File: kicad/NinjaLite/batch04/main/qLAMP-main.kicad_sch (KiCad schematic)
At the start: 19 parts, among them J3 Conn_01x07_Male, J5 Conn_01x01_Male, Q3 Q_NMOS_GSD, Q5 Q_NMOS_GSD, U17 LITE_LCD, U5 ESP32-WROOM-32

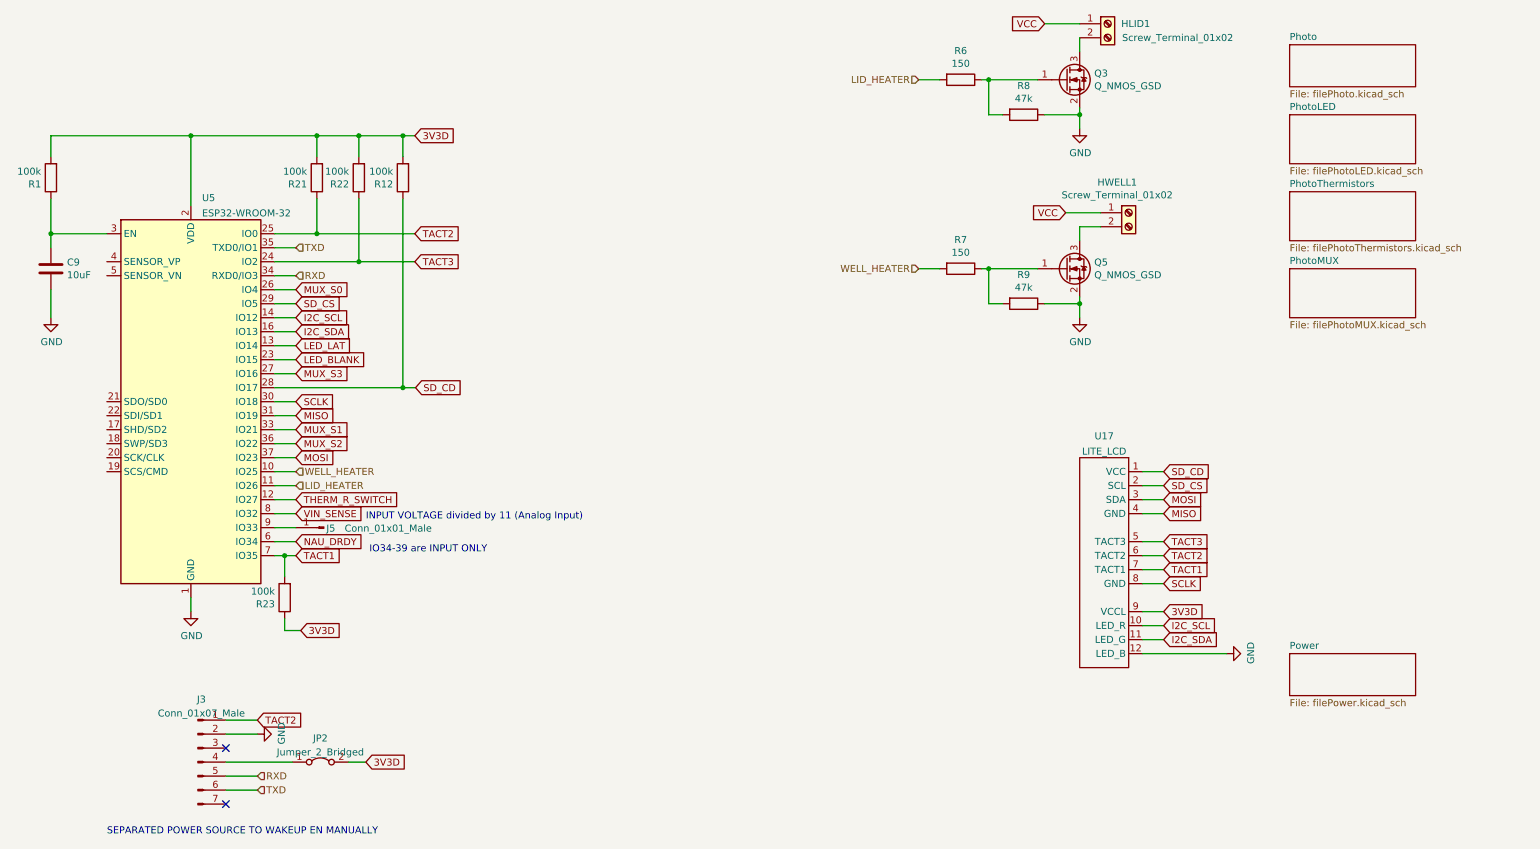
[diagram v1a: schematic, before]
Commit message: wiring batch04/main
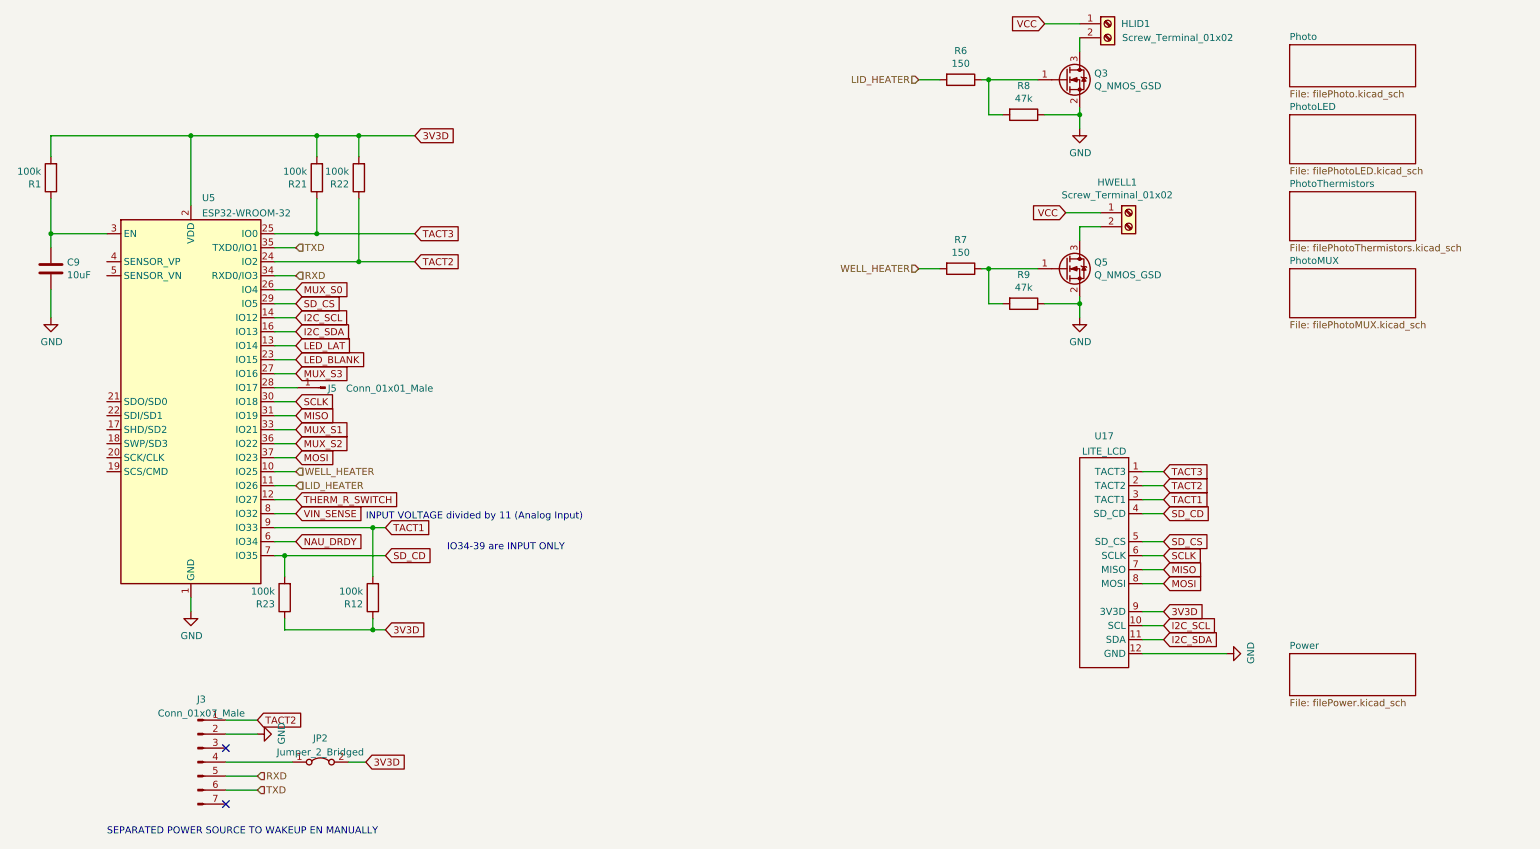
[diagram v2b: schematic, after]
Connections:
- net 3V3D: now also R12.1; no longer R12.2
- net MISO: now also U17.7 (MISO); no longer U17.4 (GND)
- net MOSI: now also U17.8 (MOSI); no longer U17.3 (SDA)
- net SCLK: now also U17.6 (SCLK); no longer U17.8 (GND)
- net SD_CD: now also R23.2, U17.4 (SD_CD), U5.7 (IO35); no longer R12.1, U17.1 (VCC), U5.28 (IO17)
- net SD_CS: now also U17.5 (SD_CS); no longer U17.2 (SCL)
- net TACT1: now also R12.2, U17.3 (TACT1), U5.9 (IO33); no longer R23.2, U17.7 (TACT1), U5.7 (IO35)
- net TACT2: now also R22.1, U17.2 (TACT2), U5.24 (IO2); no longer R21.1, U17.6 (TACT2), U5.25 (IO0)
- net TACT3: now also R21.1, U17.1 (TACT3), U5.25 (IO0); no longer R22.1, U17.5 (TACT3), U5.24 (IO2)
- net at J5.1 (Pin_1): now also U5.28 (IO17); no longer U5.9 (IO33)
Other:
- moved on the sheet: J5, R12
